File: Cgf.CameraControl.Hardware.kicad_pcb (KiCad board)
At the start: 2 copper layers, 26.5 x 55.5 mm, 30 parts, among them J1 5V input, J3 Pan, J4 Tilt, J5 SJ1-2503A, J6 Prog, J7 Sensor, Q1 BSS123, Q2 BSS123, Q4 MUN5211DW1, Q5 BSS123, U1 WT32-ETH01, U2 DRV8212DRLR, U4 DRV8212DRLR, U5 74LVC2T45DC

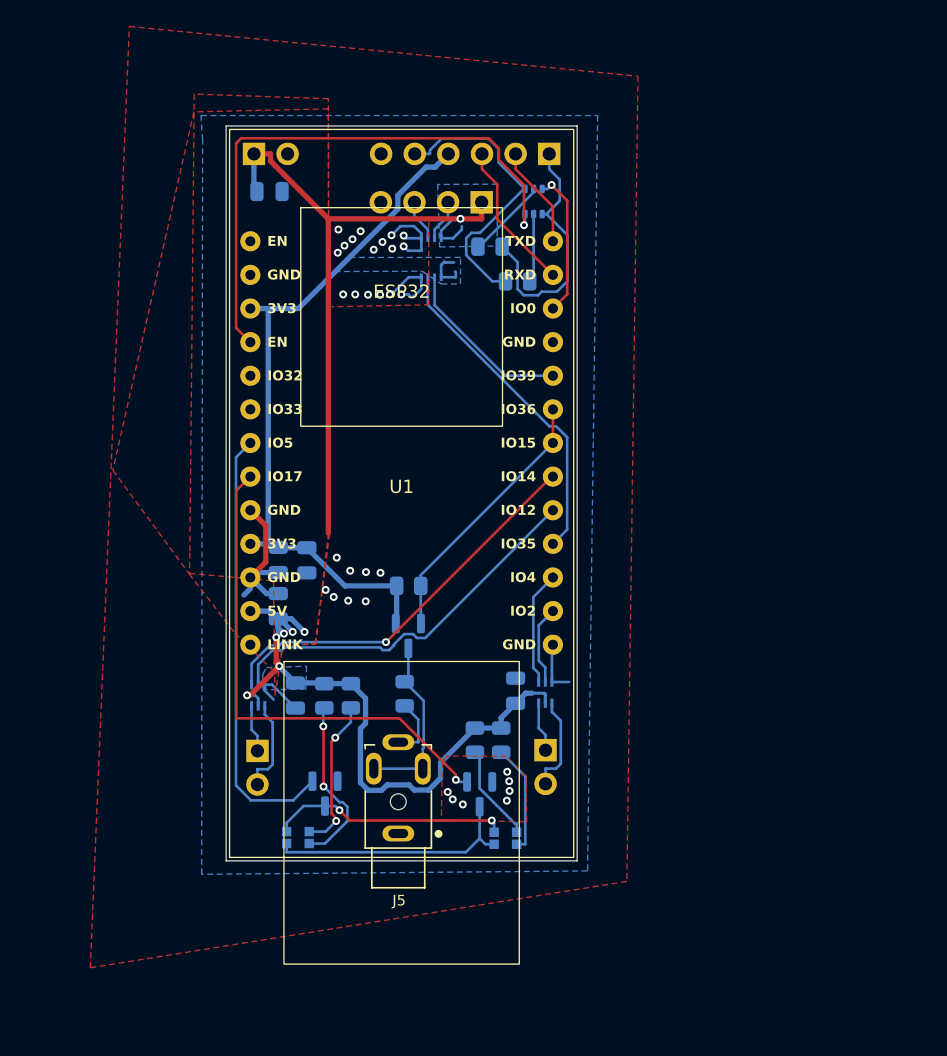
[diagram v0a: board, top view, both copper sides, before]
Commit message: improve layout
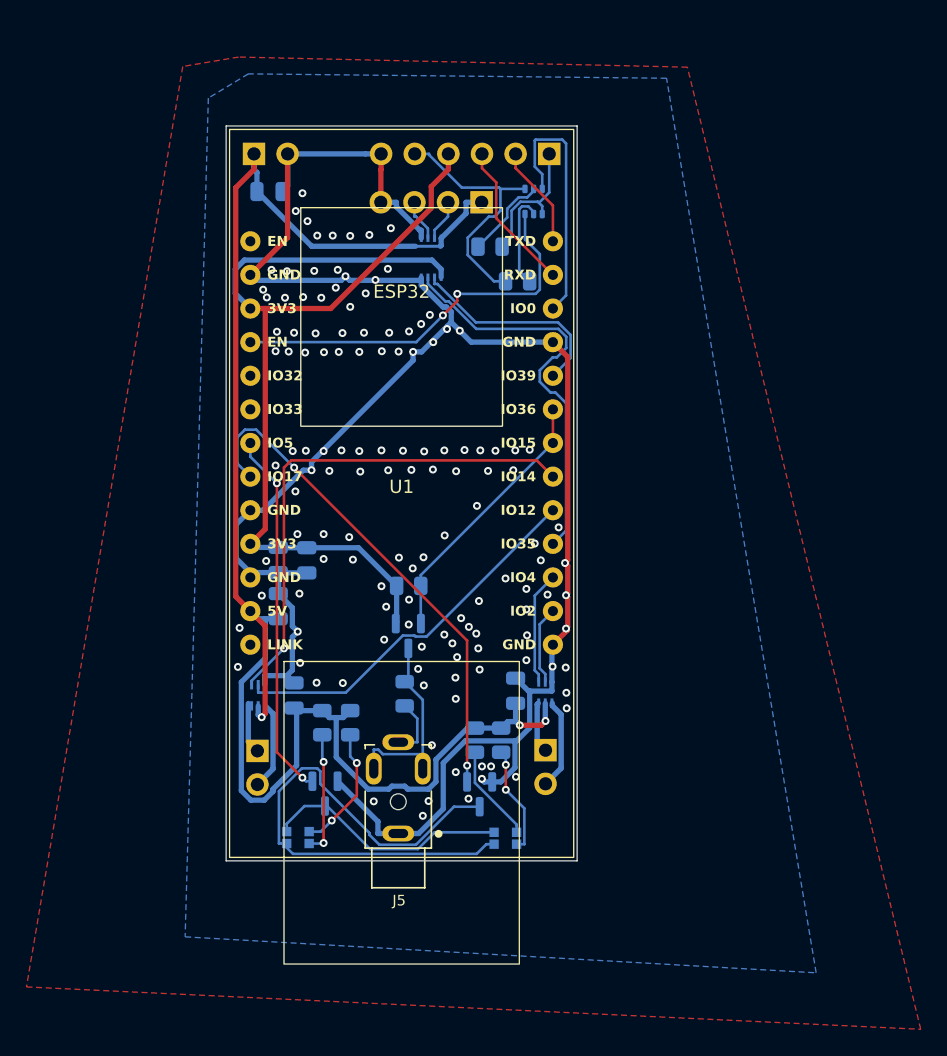
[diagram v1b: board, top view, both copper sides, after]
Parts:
- moved R3 2.04 mm to (70.7, 66.3)
- moved R5 2.03 mm to (72.8, 66.3)
- moved C5 0.10 mm to (68.6, 64.3), turned to 90 degrees
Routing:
- net GND: track 33.6 -> 160.0 mm, vias 32 -> 133
- net +5V: track 101.8 -> 125.7 mm, vias 7 -> 3
- net Net-(Q5-D): track 19.3 -> 41.2 mm
- net +3V3: track 57.0 -> 75.1 mm
- net /EN: track 43.3 -> 30.0 mm, vias 1 -> 2
- net /DTR: track 19.4 -> 10.4 mm
- net /pan forward: track 30.2 -> 38.5 mm
- net /IO0: track 11.1 -> 19.3 mm, vias 1 -> 0
- net Net-(U1-IO35/ADC1_CH7/INPUT_ONLY): track 25.2 -> 30.7 mm
- net /GREEN: track 33.2 -> 27.8 mm, vias 0 -> 2
- net Net-(D1-Pad4): track 13.1 -> 9.33 mm
- net /RTS: track 22.2 -> 19.4 mm
- net Net-(U1-IO39/ADC1_CH3/INPUT_ONLY): track 13.3 -> 16.0 mm
- net Net-(D1-Pad3): track 11.7 -> 9.52 mm
- net Net-(Q4B-B2): track 5.20 -> 7.29 mm
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- removed copper zone on B.Cu, net +3V3
- removed copper zone on B.Cu, net +5V
- removed copper zone on F.Cu, net +5V

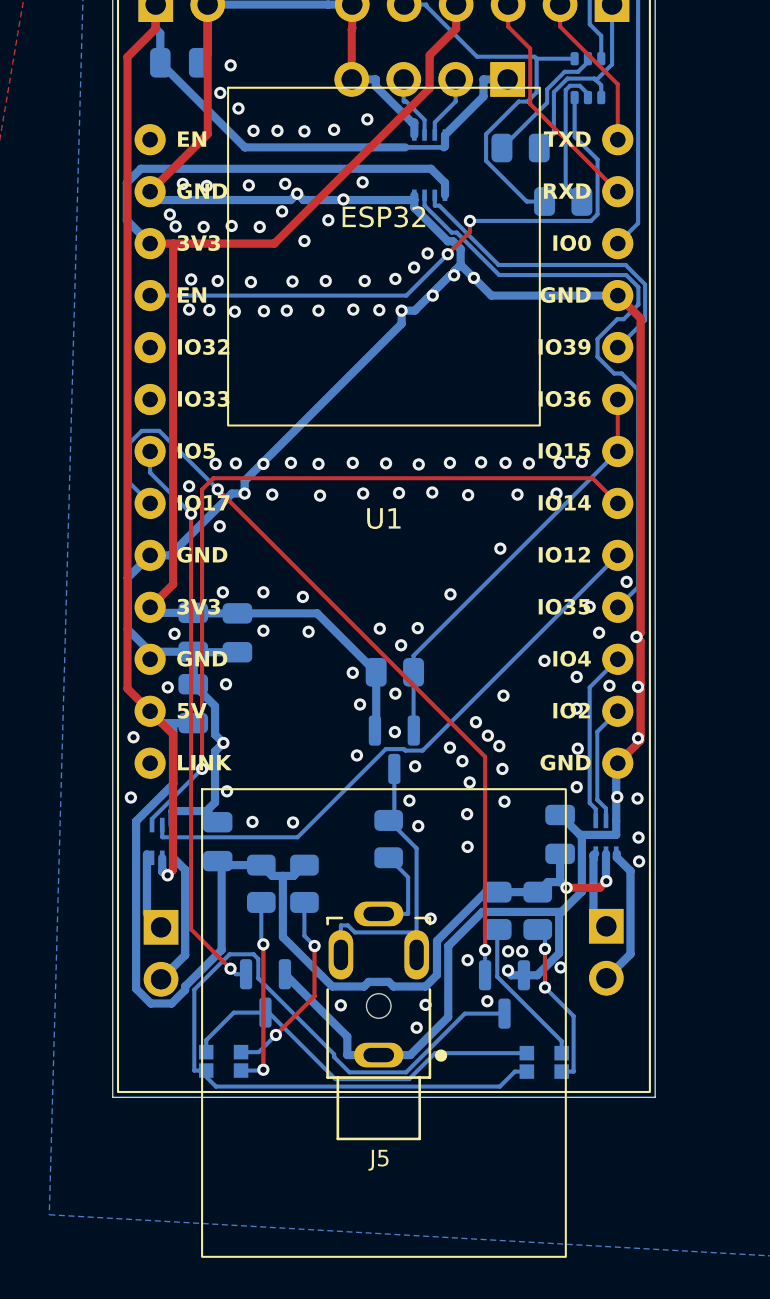
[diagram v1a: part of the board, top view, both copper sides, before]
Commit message: Fix all design rules
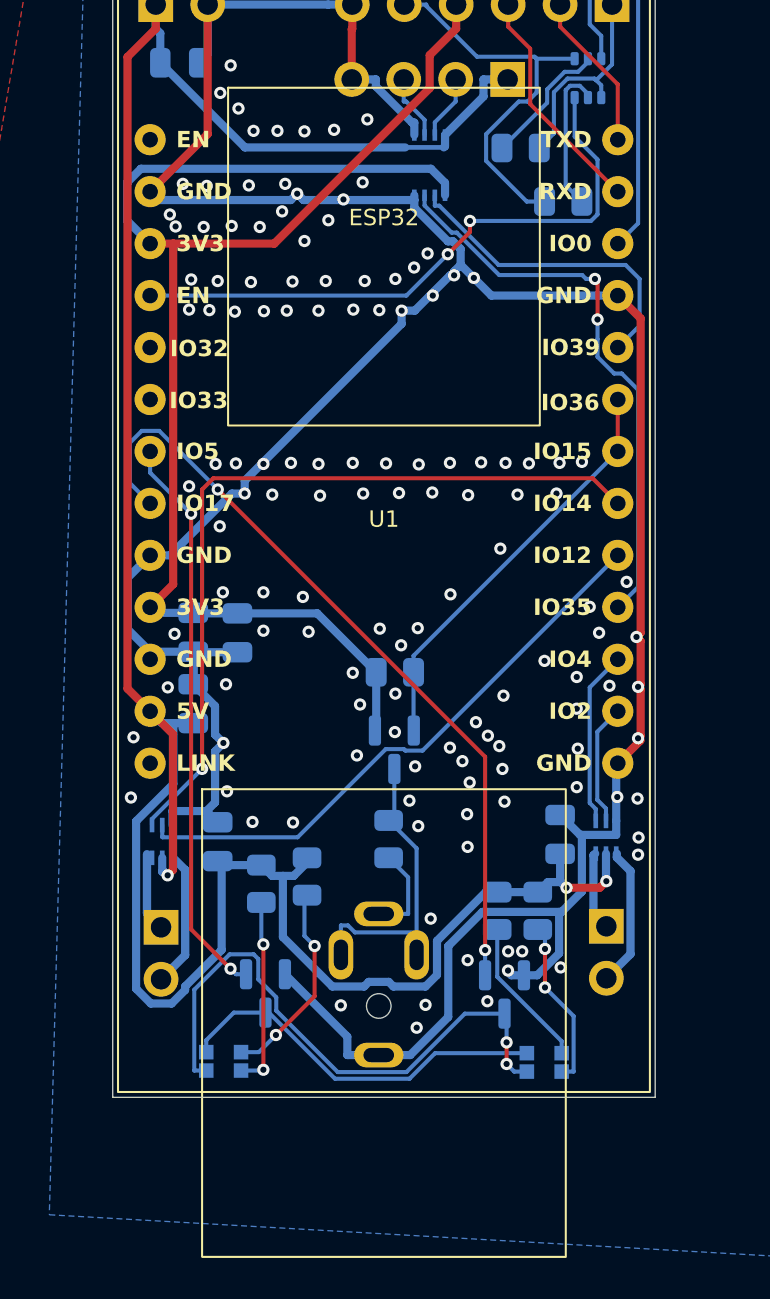
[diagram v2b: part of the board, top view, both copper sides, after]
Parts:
- J5: moved to B.Cu
- moved R5 0.38 mm to (72.9, 66.0)
- turned J5 to 0 degrees
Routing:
- net Net-(Q5-D): track 41.2 -> 28.6 mm, vias 0 -> 2
- net Net-(U1-IO35/ADC1_CH7/INPUT_ONLY): track 30.7 -> 27.9 mm, vias 0 -> 2

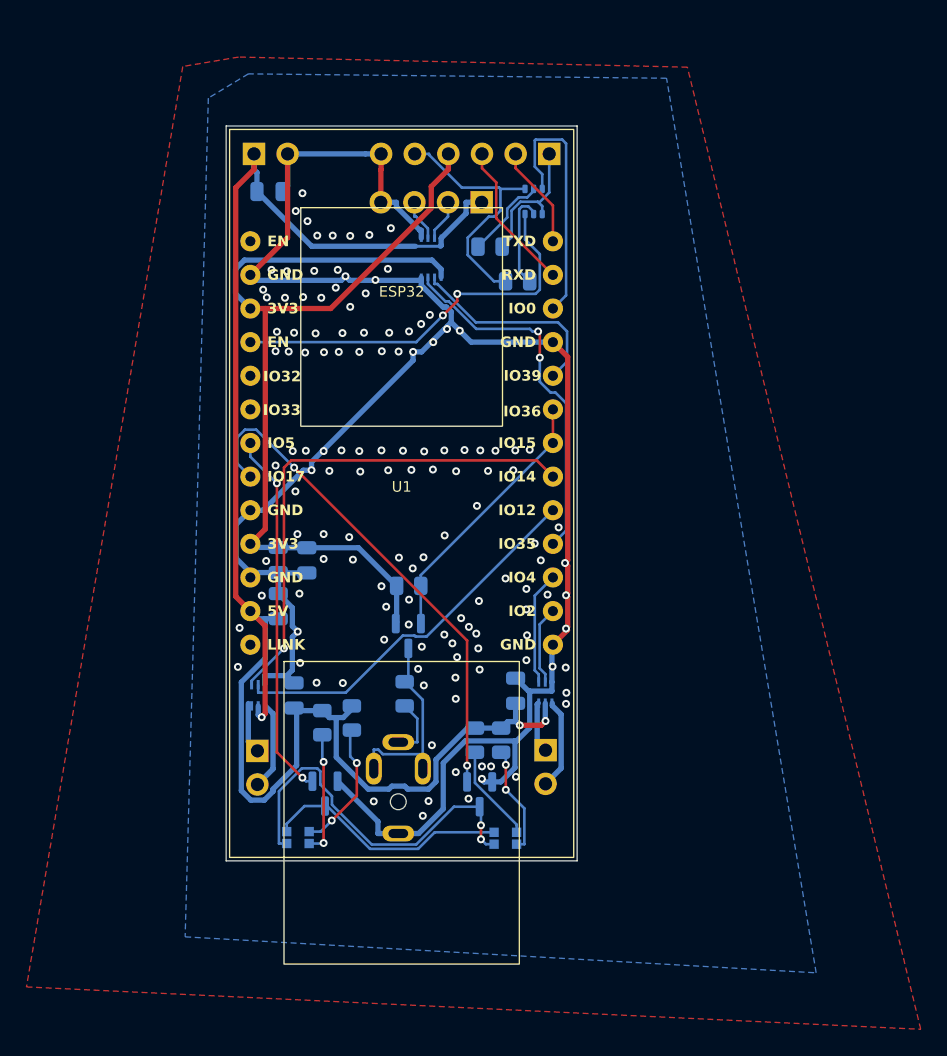
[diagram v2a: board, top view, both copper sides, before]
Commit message: improve pcb
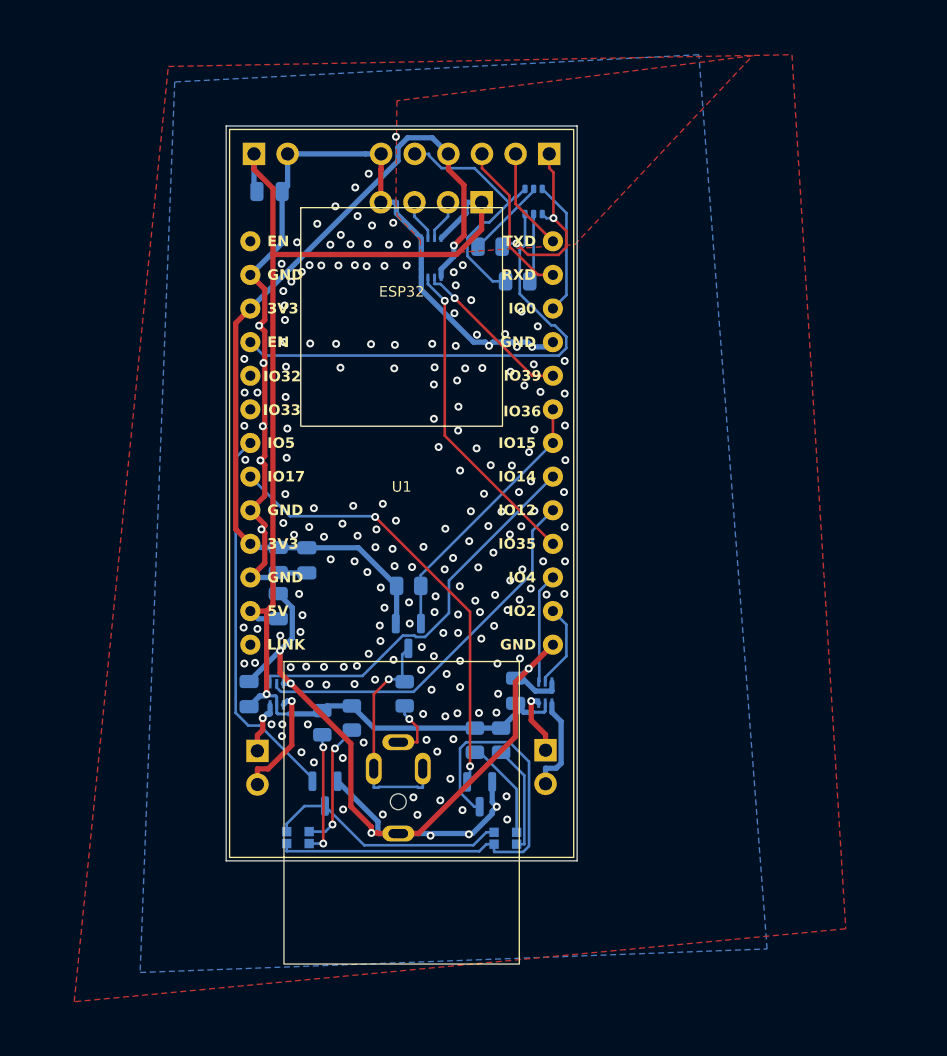
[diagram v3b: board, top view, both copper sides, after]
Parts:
- moved C5 3.41 mm to (65.2, 64.2)
- moved U4 1.40 mm to (67.3, 64.2)
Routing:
- net +5V: track 125.7 -> 98.4 mm, vias 3 -> 1
- net GND: track 160.0 -> 143.8 mm, vias 133 -> 210
- net +3V3: track 75.1 -> 65.9 mm, vias 0 -> 1
- net /IO0: track 19.3 -> 10.2 mm
- net Net-(Q5-D): track 28.6 -> 37.5 mm, vias 2 -> 0
- net /pan forward: track 38.5 -> 29.7 mm, vias 1 -> 0
- net /EN: track 30.0 -> 36.4 mm, vias 2 -> 0
- net /RED: track 38.3 -> 33.8 mm
- net Net-(U1-IO35/ADC1_CH7/INPUT_ONLY): track 27.9 -> 24.1 mm, vias 2 -> 1
- net /DTR: track 10.4 -> 14.1 mm, vias 0 -> 2
- net Net-(U1-IO39/ADC1_CH3/INPUT_ONLY): track 15.8 -> 12.3 mm, vias 0 -> 1
- net Net-(J5-tip_front): track 15.0 -> 17.7 mm, vias 0 -> 1
- net Net-(Q4B-B2): track 7.29 -> 5.20 mm
- net Net-(J3-Pin_2): track 6.67 -> 8.61 mm, vias 0 -> 1
- net /GREEN: track 27.8 -> 28.9 mm, vias 2 -> 0
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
